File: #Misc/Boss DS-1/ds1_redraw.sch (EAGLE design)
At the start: 81 parts, among them Q1 2SC732TM-GR, Q2 2SC732TM-GR, Q3 2SC732TM-GR, Q4 2SC945-P, Q5 2SC945-P, Q6 2SK30ATM-GR, Q7 2SK30ATM-Y, Q8 2SK30ATM-Y, Q9 2SC945-P

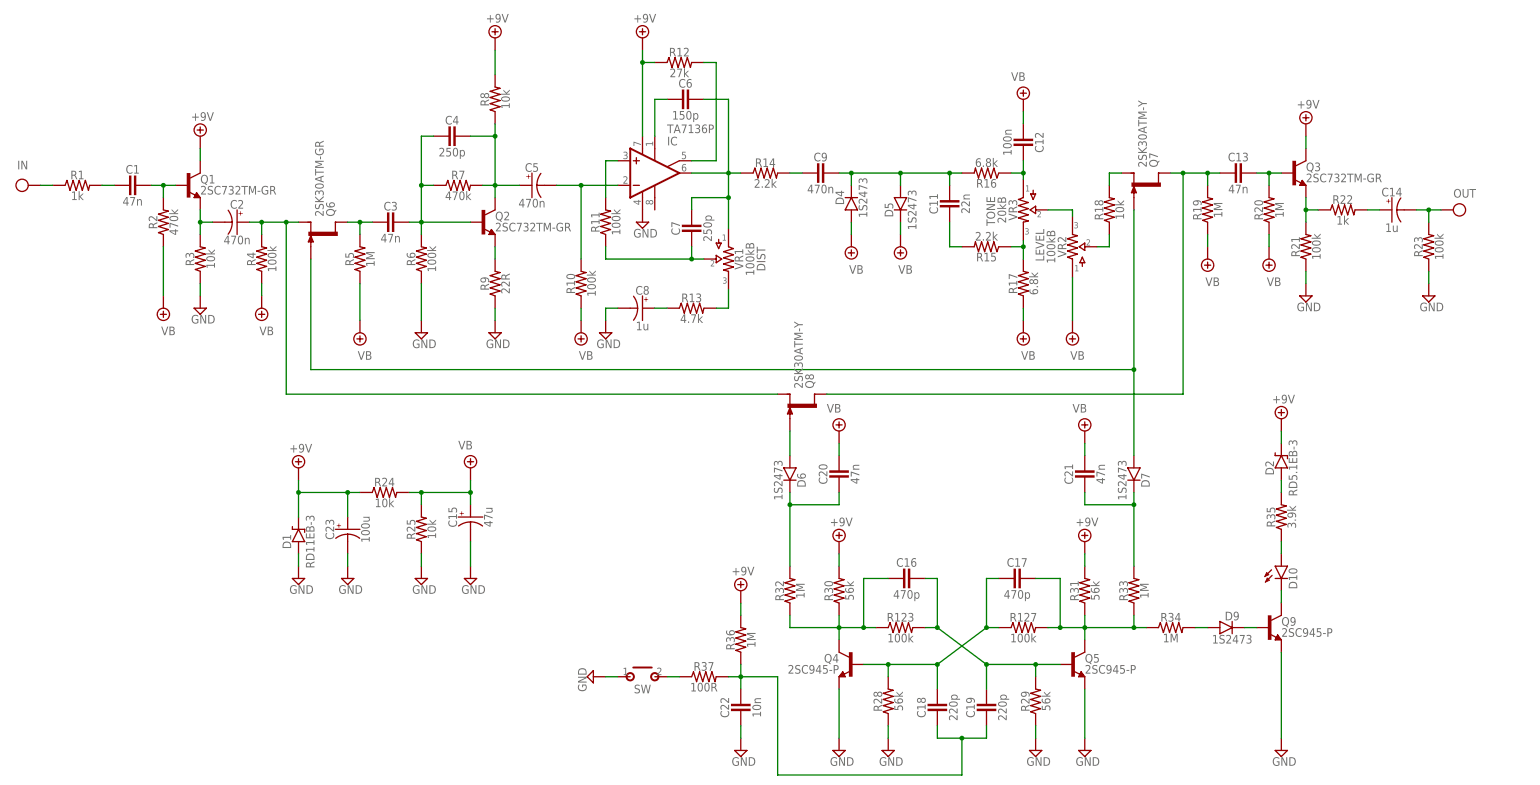
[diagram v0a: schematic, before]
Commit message: 20180529
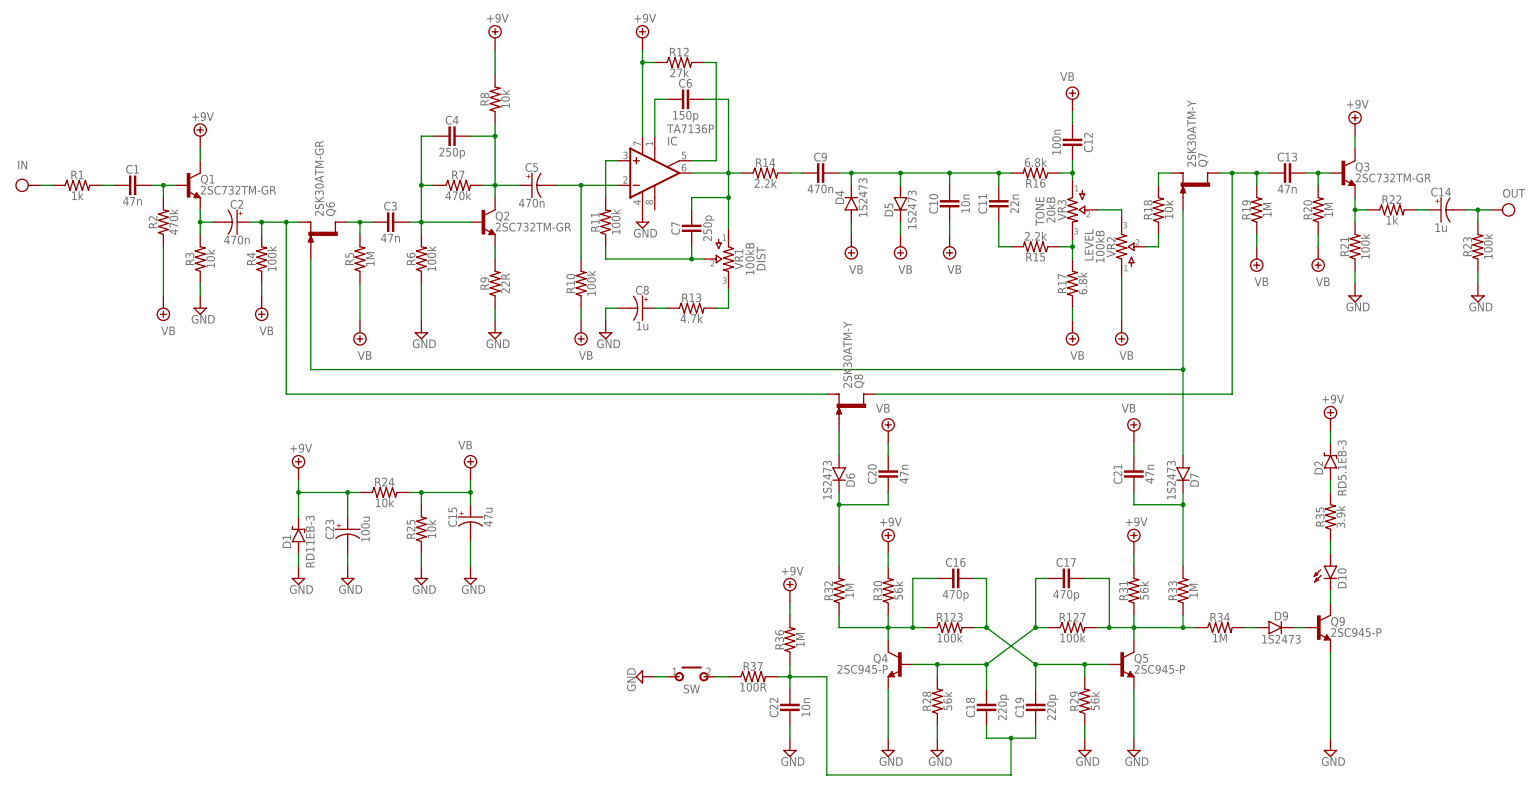
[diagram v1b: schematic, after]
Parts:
- added C10: 10n, pedals-capacitors-film:CER/FILMBOX.1
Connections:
- net N$22: now also C10.1
- net VB: now also C10.2
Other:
- moved on the sheet: C11, C12, C13, C14, C16, C17, C18, C19, C20, C21, C22, D10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
